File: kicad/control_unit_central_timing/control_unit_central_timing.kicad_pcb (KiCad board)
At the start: 2 copper layers, 25 parts

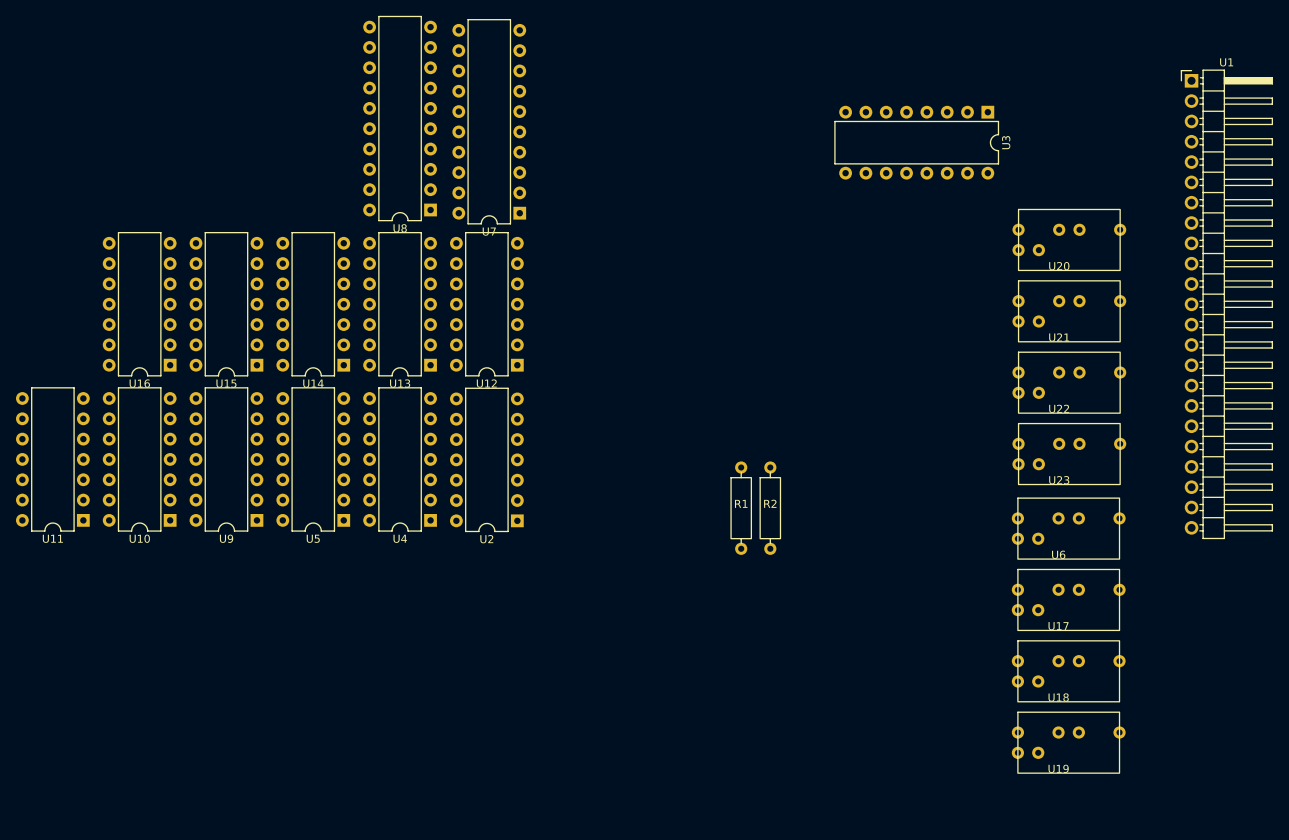
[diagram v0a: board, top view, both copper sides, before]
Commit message: Finished central timing PCB
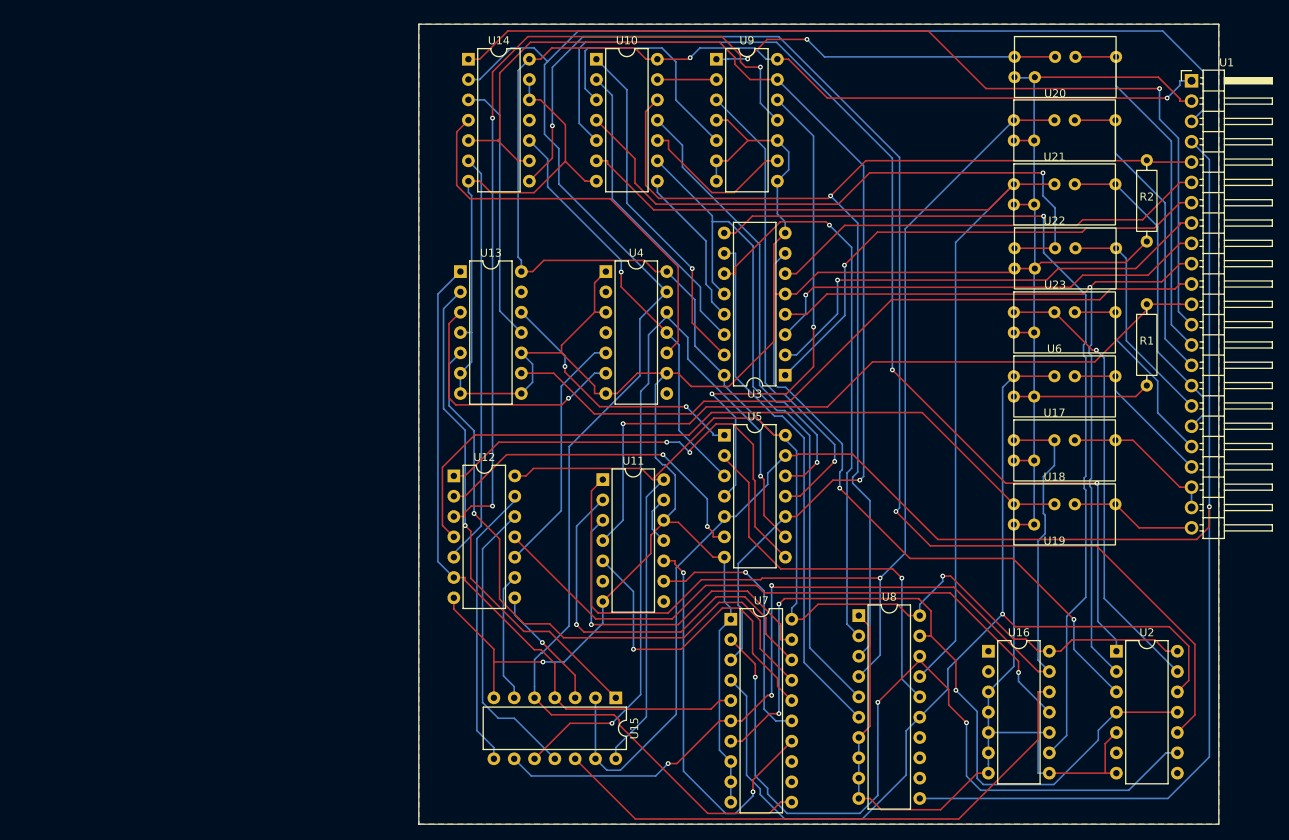
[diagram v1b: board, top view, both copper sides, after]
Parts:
- moved U16 108.3 mm to (182.2, 128.4), turned to 0 degrees
- moved U9 81.4 mm to (148.2, 54.4), turned to 0 degrees
- moved U10 78.5 mm to (133.2, 54.4), turned to 0 degrees
- moved U2 76.6 mm to (198.2, 128.4), turned to 0 degrees
- moved U8 73.7 mm to (166.0, 123.9), turned to 0 degrees
- moved U11 65.1 mm to (134.0, 106.9), turned to 0 degrees
- moved U15 61.2 mm to (135.6, 134.2), turned to -90 degrees
- moved R2 60.7 mm to (202.0, 72.1)
- moved U7 57.2 mm to (150.0, 124.4), turned to 0 degrees
- moved R1 54.7 mm to (202.0, 90.1)
- moved U5 48.8 mm to (149.2, 101.4), turned to 0 degrees
- moved U3 41.5 mm to (156.8, 93.9), turned to 180 degrees
- moved U14 41.3 mm to (117.2, 54.4), turned to 0 degrees
- moved U4 38.0 mm to (134.4, 80.9), turned to 0 degrees
- moved U19 28.5 mm to (190.5, 115.1)
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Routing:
- net Net-(U1-GND): track 0.00 -> 540.8 mm, vias 0 -> 1
- net Net-(U1-V+): track 0.00 -> 322.0 mm, vias 0 -> 3
- net Net-(U1-B_CLK): track 0.00 -> 236.8 mm, vias 0 -> 1
- net Net-(U1-A_CLK): track 0.00 -> 236.7 mm
- net Net-(U14-4Q): track 0.00 -> 167.3 mm, vias 0 -> 2
- net Net-(U14-2B): track 0.00 -> 143.0 mm, vias 0 -> 1
- net Net-(U1-BUS_MOVE_DONE): track 0.00 -> 143.0 mm, vias 0 -> 1
- net Net-(U10-1A): track 0.00 -> 137.8 mm, vias 0 -> 2
- net Net-(U11-OB): track 0.00 -> 137.3 mm, vias 0 -> 1
- net Net-(U17-IN): track 0.00 -> 129.3 mm, vias 0 -> 1
- net Net-(U10-1B): track 0.00 -> 127.7 mm
- net Net-(U15-4B): track 0.00 -> 125.8 mm, vias 0 -> 3
- net Net-(U1-BUS_READ_GOTO-DECIDER): track 0.00 -> 122.0 mm, vias 0 -> 1
- net Net-(U16-1D): track 0.00 -> 112.4 mm, vias 0 -> 1
- net Net-(U12-Q0): track 0.00 -> 104.9 mm, vias 0 -> 3
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- added copper zone on B.Cu, net Net-(U1-GND)
- added copper zone on F.Cu, net Net-(U1-V+)
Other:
- board outline added: 100 x 100 mm
